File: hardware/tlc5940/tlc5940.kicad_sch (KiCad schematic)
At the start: 21 parts, among them J1 Conn_01x06, J5 Conn_01x02, U1 TLC5940PWP

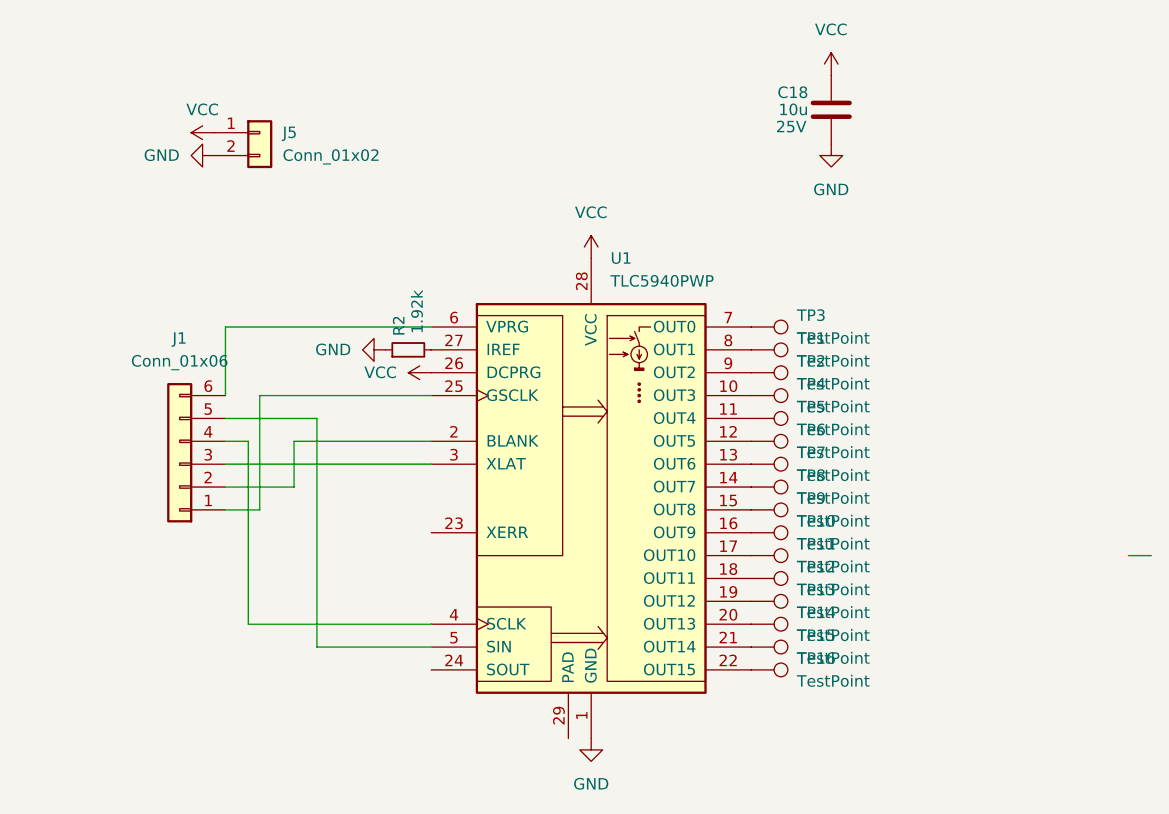
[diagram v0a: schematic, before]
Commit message: jlcpcb wip
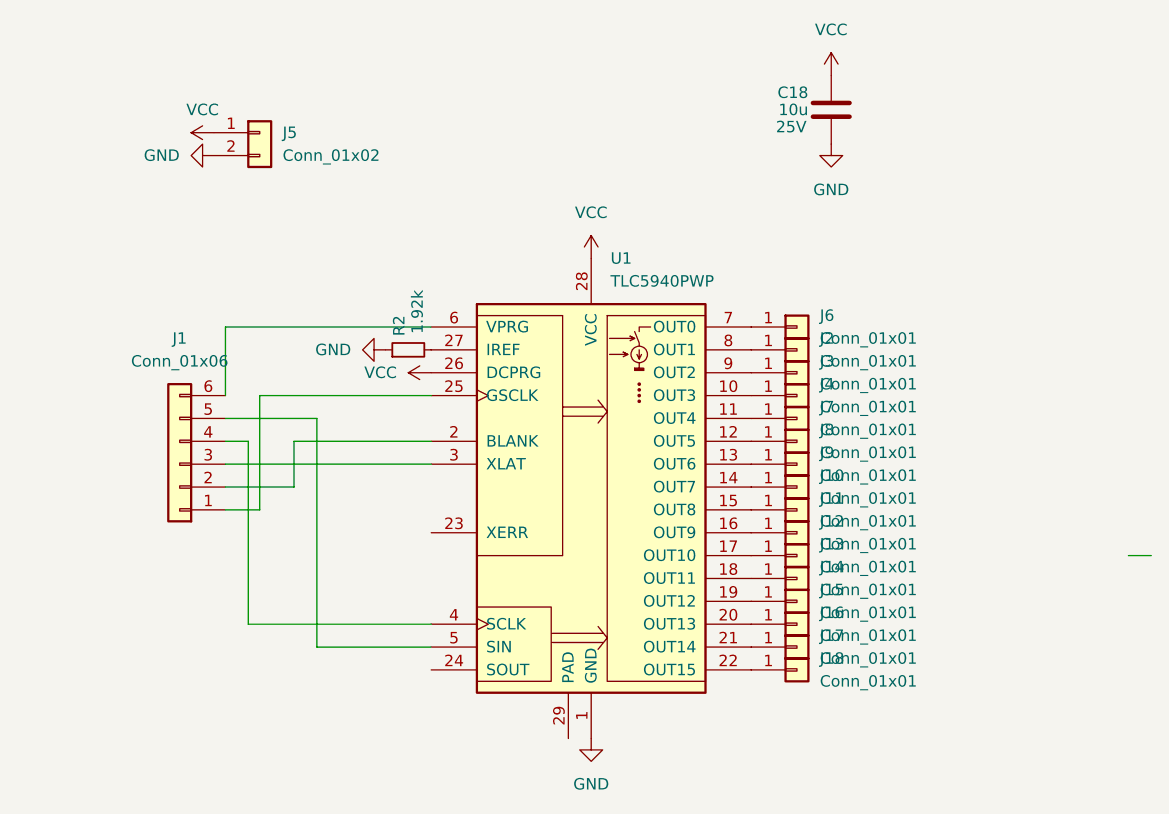
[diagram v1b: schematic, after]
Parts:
- removed TP1, TP10, TP11, TP12, TP13, TP14, TP15, TP16, TP2, TP3, TP4, TP5, TP6, TP7, TP8, TP9: TestPoint, TestPoint:TestPoint_Pad_1.0x1.0mm, symbol Connector:TestPoint
- added J10, J11, J12, J13, J14, J15, J16, J17, J18, J2, J3, J4, J6, J7, J8, J9: Conn_01x01, Connector_PinHeader_1.00mm:PinHeader_1x01_P1.00mm_Vertical, symbol Connector_Generic:Conn_01x01
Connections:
- net at U1.10 (OUT3): now also J4.1 (Pin_1)
- net at U1.11 (OUT4): now also J7.1 (Pin_1)
- net at U1.12 (OUT5): now also J8.1 (Pin_1)
- net at U1.13 (OUT6): now also J9.1 (Pin_1)
- net at U1.14 (OUT7): now also J10.1 (Pin_1)
- net at U1.15 (OUT8): now also J11.1 (Pin_1)
- net at U1.16 (OUT9): now also J12.1 (Pin_1)
- net at U1.17 (OUT10): now also J13.1 (Pin_1)
- net at U1.18 (OUT11): now also J14.1 (Pin_1)
- net at U1.19 (OUT12): now also J15.1 (Pin_1)
- net at U1.20 (OUT13): now also J16.1 (Pin_1)
- net at U1.21 (OUT14): now also J17.1 (Pin_1)
- net at U1.22 (OUT15): now also J18.1 (Pin_1)
- net at U1.7 (OUT0): now also J6.1 (Pin_1)
- net at U1.8 (OUT1): now also J2.1 (Pin_1)
- net at U1.9 (OUT2): now also J3.1 (Pin_1)

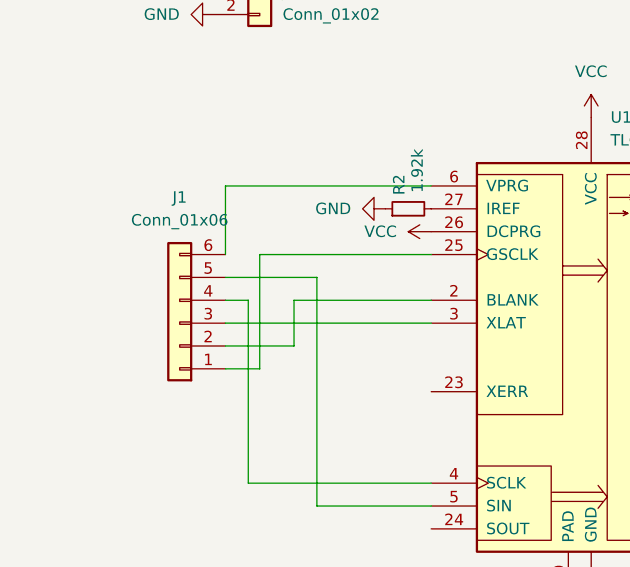
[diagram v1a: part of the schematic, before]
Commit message: wip
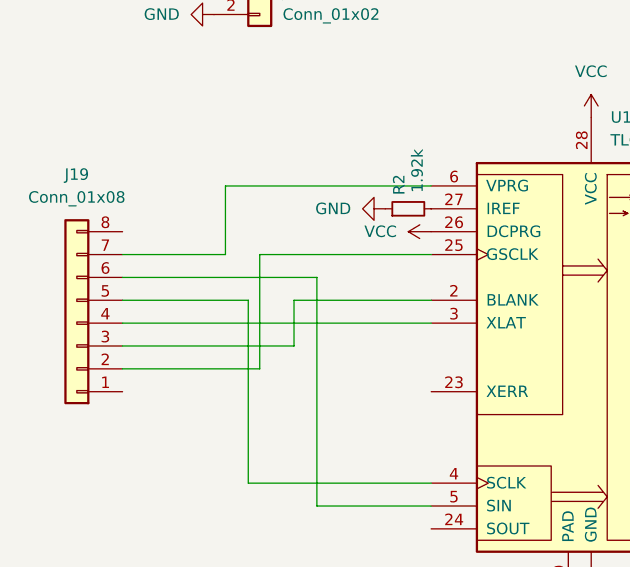
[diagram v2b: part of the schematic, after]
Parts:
- removed J1: Conn_01x06, Connector_JST:JST_SHL_SM06B-SHLS-TF_1x06-1MP_P1.00mm_Horizontal, symbol Connector_Generic:Conn_01x06
- added J19: Conn_01x08, Connector_JST:JST_SHL_SM08B-SHLS-TF_1x08-1MP_P1.00mm_Horizontal, symbol Connector_Generic:Conn_01x08
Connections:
- net at U1.2 (BLANK): now also J19.3 (Pin_3)
- net at U1.25 (GSCLK): now also J19.2 (Pin_2)
- net at U1.3 (XLAT): now also J19.4 (Pin_4)
- net at U1.4 (SCLK): now also J19.5 (Pin_5)
- net at U1.5 (SIN): now also J19.6 (Pin_6)
- net at U1.6 (VPRG): now also J19.7 (Pin_7)
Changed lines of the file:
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@@
+	(wire
+		(pts
+			(xy 87.63 60.96) (xy 99.06 60.96)
+		)
+		(stroke
+			(width 0)
+			(type default)
+		)
+	)
 	(wire
 		(pts
@@
 	(wire
 		(pts
-			(xy 106.68 66.04) (xy 106.68 71.12)
+			(xy 87.63 73.66) (xy 102.87 73.66)
 		)
 		(stroke
@@
 	(wire
 		(pts
-			(xy 106.68 66.04) (xy 121.92 66.04)
+			(xy 106.68 66.04) (xy 106.68 71.12)
 		)
 		(stroke
@@
 	(wire
 		(pts
-			(xy 101.6 66.04) (xy 99.06 66.04)
+			(xy 106.68 66.04) (xy 121.92 66.04)
 		)
 		(stroke
@@
 	(wire
 		(pts
-			(xy 199.39 78.74) (xy 201.93 78.74)
+			(xy 87.63 68.58) (xy 121.92 68.58)
 		)
 		(stroke
@@
 	(wire
 		(pts
-			(xy 99.06 60.96) (xy 99.06 53.34)
+			(xy 87.63 63.5) (xy 109.22 63.5)
 		)
 		(stroke
@@
 	(wire
 		(pts
-			(xy 99.06 63.5) (xy 109.22 63.5)
+			(xy 199.39 78.74) (xy 201.93 78.74)
 		)
 		(stroke
@@
 	(wire
 		(pts
-			(xy 101.6 86.36) (xy 101.6 66.04)
+			(xy 87.63 66.04) (xy 101.6 66.04)
 		)
 		(stroke
@@
 	(wire
 		(pts
-			(xy 106.68 71.12) (xy 99.06 71.12)
+			(xy 99.06 60.96) (xy 99.06 53.34)
 		)
 		(stroke
@@
 	(wire
 		(pts
-			(xy 99.06 68.58) (xy 121.92 68.58)
+			(xy 87.63 71.12) (xy 106.68 71.12)
 		)
 		(stroke
@@
 	(wire
 		(pts
-			(xy 102.87 73.66) (xy 99.06 73.66)
+			(xy 101.6 86.36) (xy 101.6 66.04)
 		)
 		(stroke
@@
 	)
 	(symbol
+		(lib_id "Connector_Generic:Conn_01x08")
+		(at 82.55 68.58 180)
+		(unit 1)
+		(exclude_from_sim no)
+		(in_bom yes)
+		(on_board yes)
+		(dnp no)
+		(fields_autoplaced yes)
+		(property "Reference" "J19"
+			(at 82.55 52.07 0)
+			(effects
+				(font
+					(size 1.27 1.27)
+				)
+			)
+		)
+		(property "Value" "Conn_01x08"
+			(at 82.55 54.61 0)
+			(effects
+				(font
+					(size 1.27 1.27)
+				)
+			)
+		)
+		(property "Footprint" "Connector_JST:JST_SHL_SM08B-SHLS-TF_1x08-1MP_P1.00mm_Horizontal"
+			(at 82.55 68.58 0)
+			(effects
+				(font
+					(size 1.27 1.27)
+				)
+				(hide yes)
+			)
+		)
+		(property "Datasheet" "~"
+			(at 82.55 68.58 0)
+			(effects
+				(font
+					(size 1.27 1.27)
+				)
+				(hide yes)
+			)
+		)
+		(property "Description" "Generic connector, single row, 01x08, script generated (kicad-library-utils/schlib/autogen/connector/)"
+			(at 82.55 68.58 0)
+			(effects
+				(font
+					(size 1.27 1.27)
+				)
+				(hide yes)
+			)
+		)
+		(pin "1"
+		)
+		(pin "3"
+		)
+		(pin "4"
+		)
+		(pin "2"
+		)
+		(pin "6"
+		)
+		(pin "8"
+		)
+		(pin "7"
+		)
+		(pin "5"
+		)
+		(instances
+			(project ""
+				(path "/9d64b1b8-57eb-4218-8a7c-add3e4ef813a"
+					(reference "J19")
+					(unit 1)
+				)
+			)
+		)
+	)
+	(symbol
 		(lib_id "Connector_Generic:Conn_01x01")
 		(at 162.56 88.9 0)
@@
 					(unit 1)
 				)
-			)
-		)
-	)
-	(symbol
-		(lib_id "Connector_Generic:Conn_01x06")
-		(at 93.98 68.58 180)
-		(unit 1)
-		(exclude_from_sim no)
-		(in_bom yes)
-		(on_board yes)
-		(dnp no)
-		(fields_autoplaced yes)
-		(property "Reference" "J1"
-			(at 93.98 54.61 0)
-			(effects
-				(font
-					(size 1.27 1.27)
-				)
-			)
-		)
-		(property "Value" "Conn_01x06"
-			(at 93.98 57.15 0)
-			(effects
-				(font
-					(size 1.27 1.27)
-				)
-			)
-		)
-		(property "Footprint" "Connector_JST:JST_SHL_SM06B-SHLS-TF_1x06-1MP_P1.00mm_Horizontal"
-			(at 93.98 68.58 0)
-			(effects
-				(font
-					(size 1.27 1.27)
-				)
-				(hide yes)
-			)
-		)
-		(property "Datasheet" "~"
-			(at 93.98 68.58 0)
-			(effects
-				(font
-					(size 1.27 1.27)
-				)
-				(hide yes)
-			)
-		)
-		(property "Description" "Generic connector, single row, 01x06, script generated (kicad-library-utils/schlib/autogen/connector/)"
-			(at 93.98 68.58 0)
-			(effects
-				(font
-					(size 1.27 1.27)
-				)
-				(hide yes)
-			)
-		)
-		(pin "1"
-		)
-		(pin "3"
-		)
-		(pin "2"
-		)
-		(pin "4"
-		)
-		(pin "5"
-		)
-		(pin "6"
-		)
-		(instances
-			(project ""
-				(path "/9d64b1b8-57eb-4218-8a7c-add3e4ef813a"
-					(reference "J1")
-					(unit 1)
-				)
